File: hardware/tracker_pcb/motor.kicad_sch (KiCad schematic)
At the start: 7 parts, among them IC1 DRV8244HQRYJRQ1

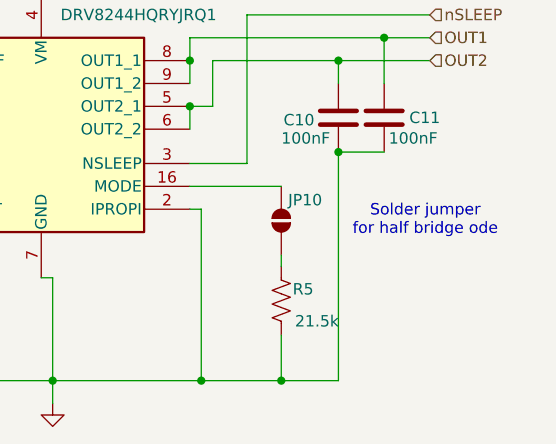
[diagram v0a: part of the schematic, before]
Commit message: WIP
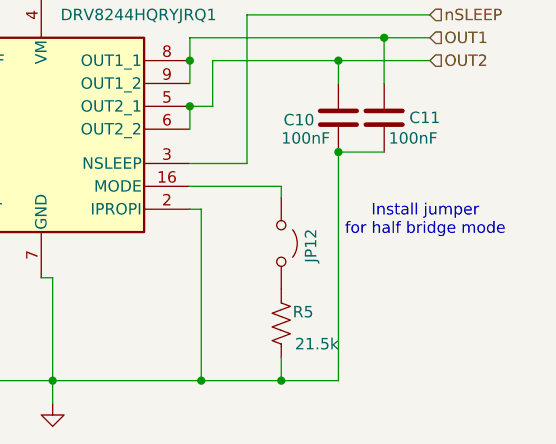
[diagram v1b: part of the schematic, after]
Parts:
- removed JP10: SolderJumper_2_Open, Resistor_SMD:R_0402_1005Metric_Pad0.72x0.64mm_HandSolder, symbol Jumper:SolderJumper_2_Open
- added JP12: Jumper_2_Open, Connector_PinHeader_2.00mm:PinHeader_1x02_P2.00mm_Vertical, symbol Jumper:Jumper_2_Open
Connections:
- net at R5.2: now also JP12.2 (B)
- net at IC1.16 (MODE): now also JP12.1 (A)
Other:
- note added: "Install jumper for half bridge mode"
- note removed: "Solder jumper for half bridge ode"
- moved on the sheet: R5
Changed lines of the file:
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@@
 	(generator_version "9.0")
 	(paper "A4")
-	(text "Solder jumper\nfor half bridge ode"
+	(text "Install jumper\nfor half bridge mode"
 		(exclude_from_sim no)
 		(at 183.642 101.6 0)
@@
 	(wire
 		(pts
-			(xy 167.64 114.3) (xy 167.64 119.38)
+			(xy 167.64 116.84) (xy 167.64 119.38)
 		)
 		(stroke
@@
 	(wire
 		(pts
-			(xy 167.64 106.68) (xy 167.64 105.41)
+			(xy 167.64 97.79) (xy 167.64 99.06)
 		)
 		(stroke
@@
 	(symbol
 		(lib_id "Device:R_US")
-		(at 167.64 110.49 180)
+		(at 167.64 113.03 180)
 		(unit 1)
 		(exclude_from_sim no)
@@
 		(dnp no)
 		(property "Reference" "R5"
-			(at 168.91 109.22 0)
+			(at 168.91 111.76 0)
 			(effects
 				(font
@@
 		)
 		(property "Value" "21.5k"
-			(at 169.164 112.776 0)
+			(at 169.164 115.316 0)
 			(effects
 				(font
@@
 		)
 		(property "Footprint" "Resistor_SMD:R_0603_1608Metric"
-			(at 166.624 110.236 90)
+			(at 166.624 112.776 90)
 			(effects
 				(font
@@
 		)
 		(property "Datasheet" "~"
-			(at 167.64 110.49 0)
+			(at 167.64 113.03 0)
 			(effects
 				(font
@@
 		)
 		(property "Description" "Resistor, US symbol"
-			(at 167.64 110.49 0)
+			(at 167.64 113.03 0)
 			(effects
 				(font
@@
 	)
 	(symbol
+		(lib_id "Jumper:Jumper_2_Open")
+		(at 167.64 104.14 270)
+		(unit 1)
+		(exclude_from_sim no)
+		(in_bom yes)
+		(on_board yes)
+		(dnp no)
+		(property "Reference" "JP12"
+			(at 170.942 104.394 0)
+			(effects
+				(font
+					(size 1.27 1.27)
+				)
+			)
+		)
+		(property "Value" "Jumper_2_Open"
+			(at 165.354 104.394 0)
+			(effects
+				(font
+					(size 1.27 1.27)
+				)
+				(hide yes)
+			)
+		)
+		(property "Footprint" "Connector_PinHeader_2.00mm:PinHeader_1x02_P2.00mm_Vertical"
+			(at 167.64 104.14 0)
+			(effects
+				(font
+					(size 1.27 1.27)
+				)
+				(hide yes)
+			)
+		)
+		(property "Datasheet" "~"
+			(at 167.64 104.14 0)
+			(effects
+				(font
+					(size 1.27 1.27)
+				)
+				(hide yes)
+			)
+		)
+		(property "Description" "Jumper, 2-pole, open"
+			(at 167.64 104.14 0)
+			(effects
+				(font
+					(size 1.27 1.27)
+				)
+				(hide yes)
+			)
+		)
+		(pin "2"
+		)
+		(pin "1"
+		)
+		(instances
+			(project "tracker_pcb"
+				(path "/6aaa9514-f94e-4843-90d0-16960e4e49cb/7a9ac5e6-2be9-4d8c-8c5b-8ceb68264255"
+					(reference "JP12")
+					(unit 1)
+				)
+				(path "/6aaa9514-f94e-4843-90d0-16960e4e49cb/f8a23924-a799-4920-a190-8ed5e6a03d20"
+					(reference "JP13")
+					(unit 1)
+				)
+			)
+		)
+	)
+	(symbol
 		(lib_id "Device:C")
 		(at 179.07 90.17 0)
@@
 					(unit 1)
 				)
-			)
-		)
-	)
-	(symbol
-		(lib_id "Jumper:SolderJumper_2_Open")
-		(at 167.64 101.6 90)
-		(unit 1)
-		(exclude_from_sim no)
-		(in_bom no)
-		(on_board yes)
-		(dnp no)
-		(property "Reference" "JP10"
-			(at 168.402 99.314 90)
-			(effects
-				(font
-					(size 1.27 1.27)
-				)
-				(justify right)
-			)
-		)
-		(property "Value" "SolderJumper_2_Open"
-			(at 163.83 101.6 0)
-			(effects
-				(font
-					(size 1.27 1.27)
-				)
-				(hide yes)
-			)
-		)
-		(property "Footprint" "Resistor_SMD:R_0402_1005Metric_Pad0.72x0.64mm_HandSolder"
-			(at 167.64 101.6 0)
-			(effects
-				(font
-					(size 1.27 1.27)
-				)
-				(hide yes)
-			)
-		)
-		(property "Datasheet" "~"
-			(at 167.64 101.6 0)
-			(effects
-				(font
-					(size 1.27 1.27)
-				)
-				(hide yes)
-			)
-		)
-		(property "Description" "Solder Jumper, 2-pole, open"
-			(at 167.64 101.6 0)
-			(effects
-				(font
-					(size 1.27 1.27)
-				)
-				(hide yes)
-			)
-		)
-		(pin "2"
-		)
-		(pin "1"
-		)
-		(instances
-			(project "tracker_pcb"
-				(path "/6aaa9514-f94e-4843-90d0-16960e4e49cb/7a9ac5e6-2be9-4d8c-8c5b-8ceb68264255"
-					(reference "JP10")
-					(unit 1)
-				)
-				(path "/6aaa9514-f94e-4843-90d0-16960e4e49cb/f8a23924-a799-4920-a190-8ed5e6a03d20"
-					(reference "JP11")
-					(unit 1)
-				)

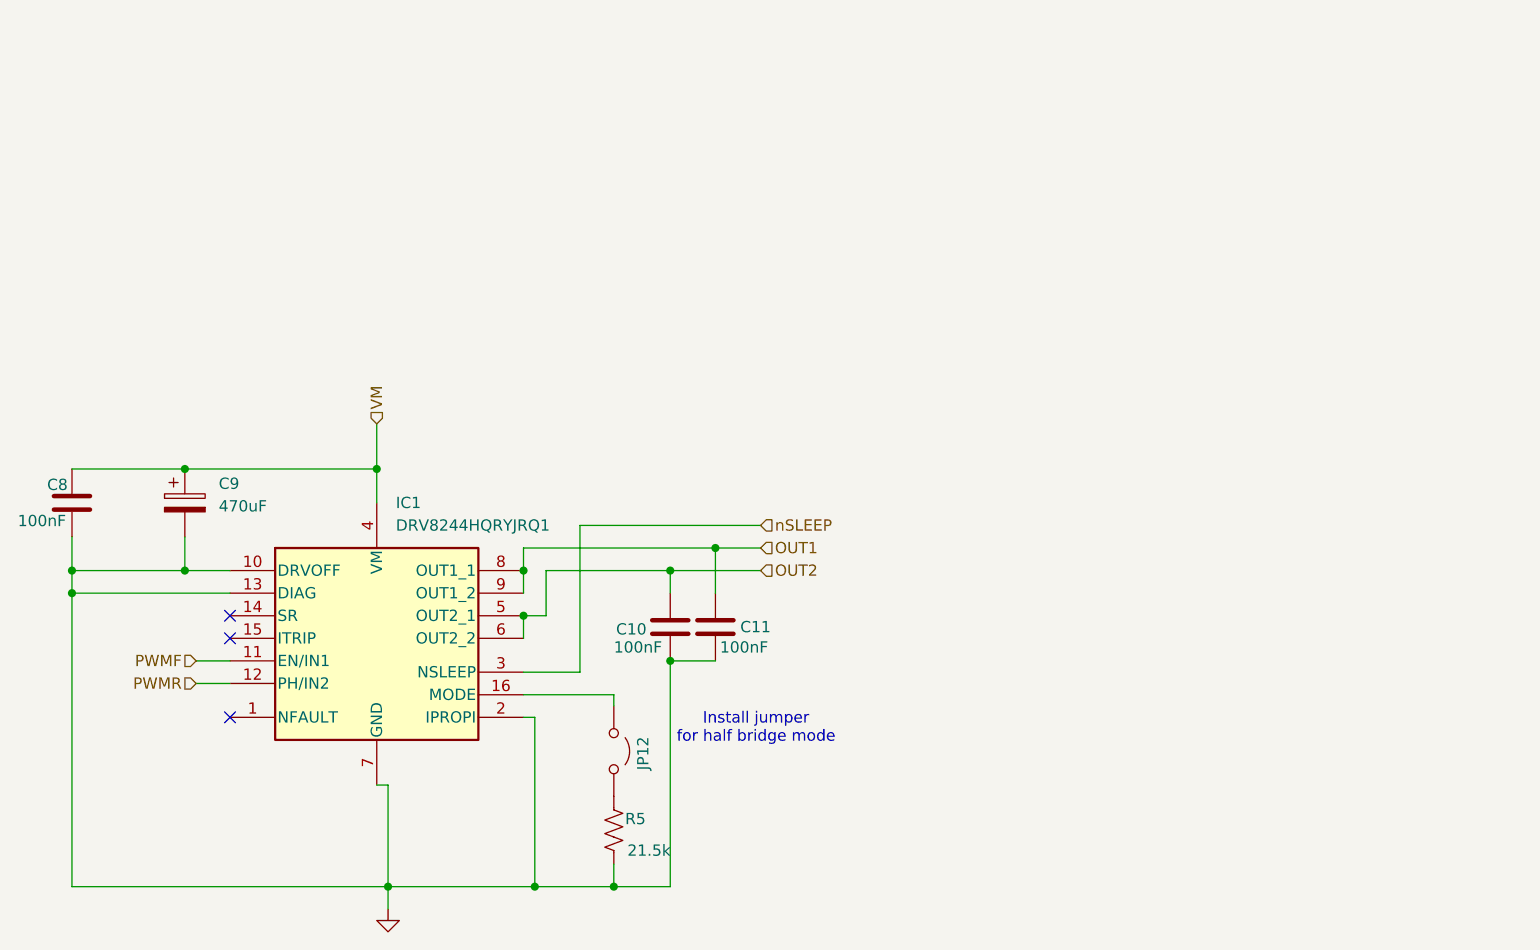
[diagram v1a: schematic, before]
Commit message: Including LORA wio-sx1262
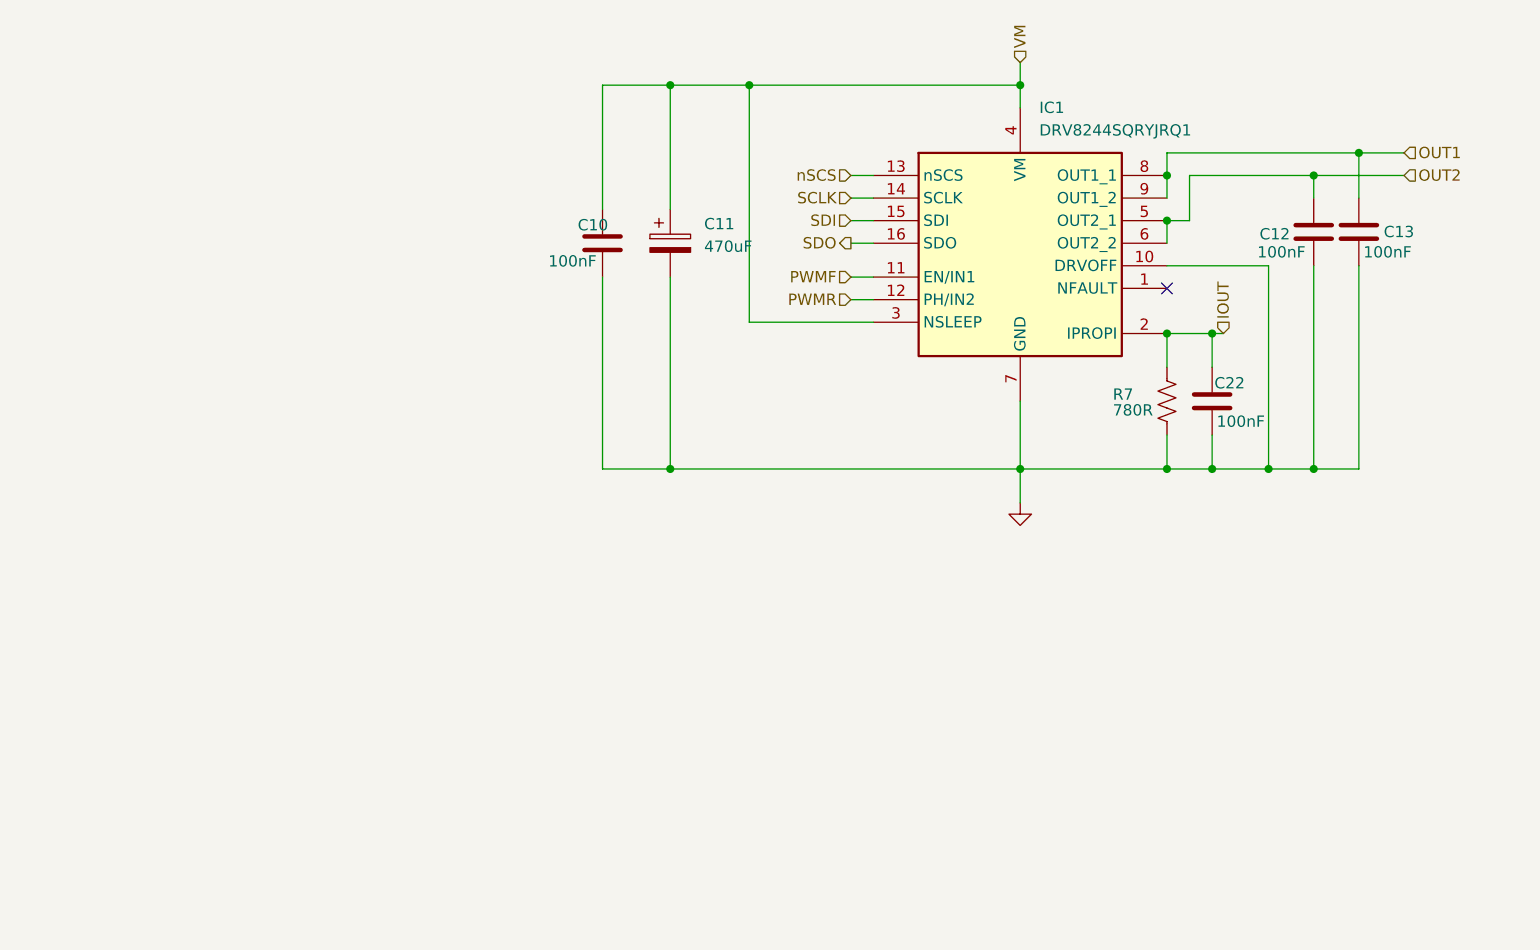
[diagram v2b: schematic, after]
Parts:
- removed IC1: DRV8244HQRYJRQ1, RXZ0016A-MFG, symbol symbol:DRV8245HQRXZRQ1
- removed JP12: Jumper_2_Open, Connector_PinHeader_2.00mm:PinHeader_1x02_P2.00mm_Vertical, symbol Jumper:Jumper_2_Open
- removed R5: 21.5k, Resistor_SMD:R_0603_1608Metric, symbol Device:R_US
- added C22: 100nF, Capacitor_SMD:C_0603_1608Metric, symbol Device:C
- added IC1: DRV8244SQRYJRQ1, footprint:DRV8244HQRYJRQ1, symbol symbol:DRV8244SQRYJRQ1
- added R7: 780R, Resistor_SMD:R_0603_1608Metric, symbol Device:R_US
- C10: renamed from C8; LCSC (none) -> C1590
- C11: renamed from C9; LCSC (none) -> C688951
- C12: renamed from C10; LCSC (none) -> C1590
- C13: renamed from C11; LCSC (none) -> C1590
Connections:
- net GND: now also C22.2, IC1.10 (DRVOFF), IC1.7 (GND), R7.1
- net OUT1: now also IC1.8 (OUT1_1), IC1.9 (OUT1_2)
- net OUT2: now also IC1.5 (OUT2_1), IC1.6 (OUT2_2)
- net PWMF: now also IC1.11 (EN/IN1)
- net PWMR: now also IC1.12 (PH/IN2)
- net VM: now also IC1.3 (NSLEEP), IC1.4 (VM)
- new net IOUT: C22.1, IC1.2 (IPROPI), R7.2
- new net SCLK: IC1.14 (SCLK)
- new net SDI: IC1.15 (SDI)
- new net SDO: IC1.16 (SDO)
- new net nSCS: IC1.13 (nSCS)
- no-connect marks 3 -> 1
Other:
- note removed: "Install jumper for half bridge mode"
- moved on the sheet: C10, C11, C12, C13

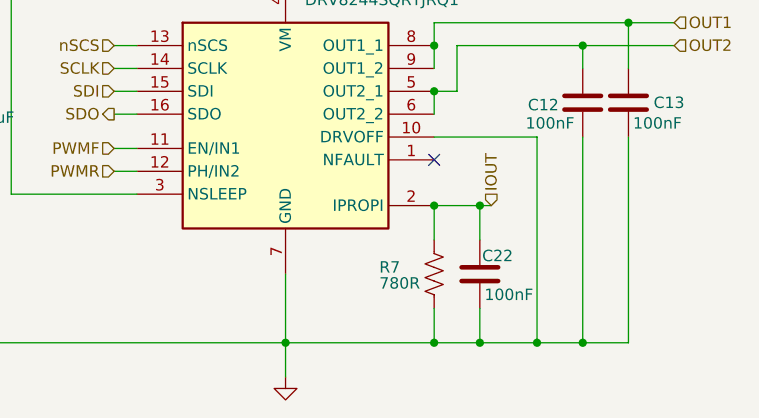
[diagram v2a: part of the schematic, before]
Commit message: VIA changes
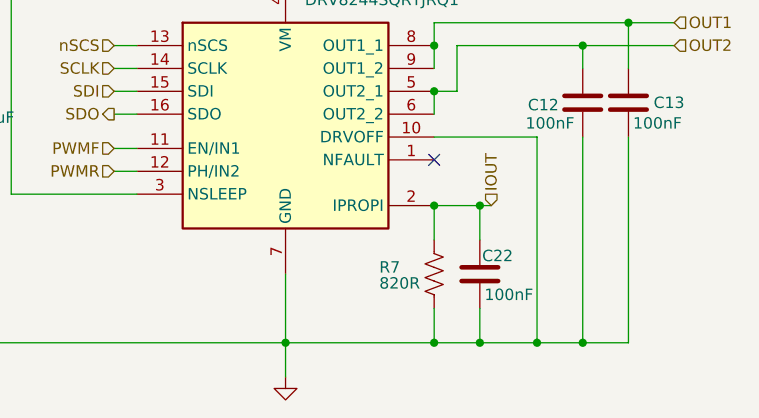
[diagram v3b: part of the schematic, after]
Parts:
- R7: value 780R -> 820R; LCSC (none) -> C23253
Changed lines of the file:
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@@
 			)
 		)
-		(property "Value" "780R"
+		(property "Value" "820R"
 			(at 223.774 65.786 0)
 			(effects
@@
 			(effects
 				(font
+					(size 1.27 1.27)
+				)
+				(hide yes)
+			)
+		)
+		(property "LCSC" "C23253"
+			(at 223.774 64.008 0)
+			(effects
+				(font

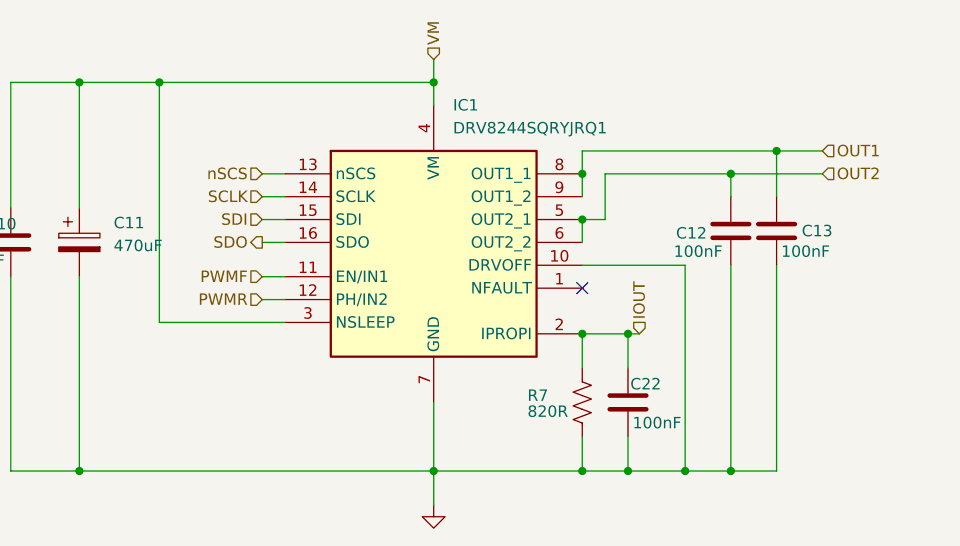
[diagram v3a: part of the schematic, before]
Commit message: ss changes
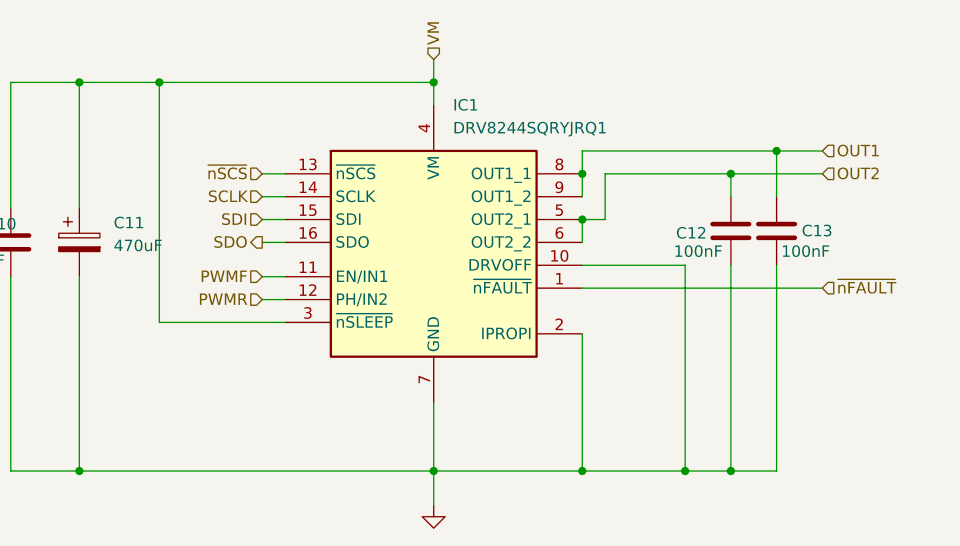
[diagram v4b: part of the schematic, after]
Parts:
- removed C22: 100nF, Capacitor_SMD:C_0603_1608Metric, symbol Device:C
- removed R7: 820R, Resistor_SMD:R_0603_1608Metric, symbol Device:R_US
- IC1: footprint footprint:DRV8244HQRYJRQ1 -> DRV8244HQRYJRQ1
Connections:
- net IOUT is gone; now on net GND: IC1.2 (IPROPI)
- net ~{nFAULT}: now reaches IC1.1 (~{nFAULT})
- net nSCS renamed ~{nSCS}
- no-connect marks 1 -> 0
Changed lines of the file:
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@@
-	)
-	(junction
-		(at 229.87 57.15)
-		(diameter 0)
-		(color 0 0 0 0)
 	)
 	(junction
@@
 	)
 	(junction
-		(at 234.95 57.15)
-		(diameter 0)
-		(color 0 0 0 0)
-	)
-	(junction
 		(at 213.36 29.21)
 		(diameter 0)
@@
 	)
 	(junction
-		(at 234.95 72.39)
-		(diameter 0)
-		(color 0 0 0 0)
-	)
-	(junction
 		(at 241.3 72.39)
 		(diameter 0)
 		(color 0 0 0 0)
 	)
-	(no_connect
-		(at 229.87 52.07)
-	)
 	(wire
 		(pts
@@
 	(wire
 		(pts
+			(xy 229.87 57.15) (xy 229.87 72.39)
+		)
+		(stroke
+			(width 0)
+			(type default)
+		)
+	)
+	(wire
+		(pts
 			(xy 246.38 49.53) (xy 246.38 72.39)
 		)
@@
 	(wire
 		(pts
-			(xy 234.95 57.15) (xy 236.22 57.15)
-		)
-		(stroke
-			(width 0)
-			(type default)
-		)
-	)
-	(wire
-		(pts
-			(xy 229.87 57.15) (xy 229.87 60.96)
-		)
-		(stroke
-			(width 0)
-			(type default)
-		)
-	)
-	(wire
-		(pts
 			(xy 246.38 72.39) (xy 251.46 72.39)
 		)
@@
 	(wire
 		(pts
-			(xy 229.87 68.58) (xy 229.87 72.39)
-		)
-		(stroke
-			(width 0)
-			(type default)
-		)
-	)
-	(wire
-		(pts
 			(xy 251.46 49.53) (xy 251.46 72.39)
 		)
@@
 	(wire
 		(pts
-			(xy 234.95 72.39) (xy 229.87 72.39)
-		)
-		(stroke
-			(width 0)
-			(type default)
-		)
-	)
-	(wire
-		(pts
 			(xy 166.37 29.21) (xy 173.99 29.21)
 		)
@@
 	(wire
 		(pts
-			(xy 234.95 57.15) (xy 234.95 60.96)
-		)
-		(stroke
-			(width 0)
-			(type default)
-		)
-	)
-	(wire
-		(pts
 			(xy 194.31 41.91) (xy 196.85 41.91)
 		)
@@
 	(wire
 		(pts
+			(xy 229.87 52.07) (xy 256.54 52.07)
+		)
+		(stroke
+			(width 0)
+			(type default)
+		)
+	)
+	(wire
+		(pts
 			(xy 229.87 72.39) (xy 213.36 72.39)
 		)
@@
 	(wire
 		(pts
-			(xy 229.87 57.15) (xy 234.95 57.15)
-		)
-		(stroke
-			(width 0)
-			(type default)
-		)
-	)
-	(wire
-		(pts
 			(xy 194.31 46.99) (xy 196.85 46.99)
 		)
@@
 	(wire
 		(pts
-			(xy 234.95 68.58) (xy 234.95 72.39)
-		)
-		(stroke
-			(width 0)
-			(type default)
-		)
-	)
-	(wire
-		(pts
 			(xy 182.88 55.88) (xy 196.85 55.88)
 		)
@@
 	(wire
 		(pts
-			(xy 241.3 72.39) (xy 234.95 72.39)
+			(xy 229.87 72.39) (xy 241.3 72.39)
 		)
 		(stroke
@@
 		)
 	)
-	(hierarchical_label "IOUT"
-		(shape input)
-		(at 236.22 57.15 90)
-		(effects
-			(font
-				(size 1.27 1.27)
-			)
-			(justify left)
-		)
-	)
-	(hierarchical_label "nSCS"
+	(hierarchical_label "~{nSCS}"
 		(shape input)
 		(at 194.31 39.37 180)
@@
 		(shape input)
 		(at 256.54 36.83 0)
+		(effects
+			(font
+				(size 1.27 1.27)
+			)
+			(justify left)
+		)
+	)
+	(hierarchical_label "~{nFAULT}"
+		(shape input)
+		(at 256.54 52.07 0)
 		(effects
 			(font
@@
 			)
 		)
-		(property "Footprint" "footprint:DRV8244HQRYJRQ1"
+		(property "Footprint" "DRV8244HQRYJRQ1"
 			(at 226.06 134.29 0)
 			(effects
@@
 					(unit 1)
 				)
-			)
-		)
-	)
-	(symbol
-		(lib_id "Device:R_US")
-		(at 229.87 64.77 180)
-		(unit 1)
-		(exclude_from_sim no)
-		(in_bom yes)
-		(on_board yes)
-		(dnp no)
-		(property "Reference" "R7"
-			(at 223.774 64.008 0)
-			(effects
-				(font
-					(size 1.27 1.27)
-				)
-				(justify right)
-			)
-		)
-		(property "Value" "820R"
-			(at 223.774 65.786 0)
-			(effects
-				(font
-					(size 1.27 1.27)
-				)
-				(justify right)
-			)
-		)
-		(property "Footprint" "Resistor_SMD:R_0603_1608Metric"
-			(at 228.854 64.516 90)
-			(effects
-				(font
-					(size 1.27 1.27)
-				)
-				(hide yes)
-			)
-		)
-		(property "Datasheet" "~"
-			(at 229.87 64.77 0)
-			(effects
-				(font
-					(size 1.27 1.27)
-				)
-				(hide yes)
-			)
-		)
-		(property "Description" "Resistor, US symbol"
-			(at 229.87 64.77 0)
-			(effects
-				(font
-					(size 1.27 1.27)
-				)
-				(hide yes)
-			)
-		)
-		(property "LCSC" "C23253"
-			(at 223.774 64.008 0)
-			(effects
-				(font
-					(size 1.27 1.27)
-				)
-				(hide yes)
-			)
-		)
-		(pin "1"
-		)
-		(pin "2"
-		)
-		(instances
-			(project "tracker_pcb"
-				(path "/6aaa9514-f94e-4843-90d0-16960e4e49cb/7a9ac5e6-2be9-4d8c-8c5b-8ceb68264255"
-					(reference "R7")
-					(unit 1)
-				)
-				(path "/6aaa9514-f94e-4843-90d0-16960e4e49cb/f8a23924-a799-4920-a190-8ed5e6a03d20"
-					(reference "R8")
-					(unit 1)
-				)
-			)
-		)
-	)
-	(symbol
-		(lib_id "Device:C")
-		(at 234.95 64.77 0)
-		(unit 1)
-		(exclude_from_sim no)
-		(in_bom yes)
-		(on_board yes)
-		(dnp no)
-		(property "Reference" "C22"
-			(at 235.204 62.738 0)
-			(effects
-				(font
-					(size 1.27 1.27)
-				)
-				(justify left)
-			)
-		)
-		(property "Value" "100nF"
-			(at 235.458 67.056 0)
-			(effects
-				(font
-					(size 1.27 1.27)
-				)
-				(justify left)
-			)
-		)
-		(property "Footprint" "Capacitor_SMD:C_0603_1608Metric"
-			(at 235.9152 68.58 0)
-			(effects
-				(font
-					(size 1.27 1.27)
-				)
-				(hide yes)
-			)
-		)
-		(property "Datasheet" "~"
-			(at 234.95 64.77 0)
-			(effects
-				(font
-					(size 1.27 1.27)
-				)
-				(hide yes)
-			)
-		)
-		(property "Description" "Unpolarized capacitor"
-			(at 234.95 64.77 0)
-			(effects
-				(font
-					(size 1.27 1.27)
-				)
-				(hide yes)
-			)
-		)
-		(property "LCSC" "C1590"
-			(at 235.204 62.738 0)
-			(effects
-				(font
-					(size 1.27 1.27)
-				)
-				(hide yes)
-			)
-		)
-		(pin "2"
-		)
-		(pin "1"
-		)
-		(instances
-			(project "tracker_pcb"
-				(path "/6aaa9514-f94e-4843-90d0-16960e4e49cb/7a9ac5e6-2be9-4d8c-8c5b-8ceb68264255"
-					(reference "C22")
-					(unit 1)
-				)
-				(path "/6aaa9514-f94e-4843-90d0-16960e4e49cb/f8a23924-a799-4920-a190-8ed5e6a03d20"
-					(reference "C23")
-					(unit 1)
-				)
